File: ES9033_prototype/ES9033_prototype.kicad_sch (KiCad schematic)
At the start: 8 parts, among them J101 Conn_01x02, J102 Conn_01x04, J103 Conn_01x04, J104 Conn_01x04

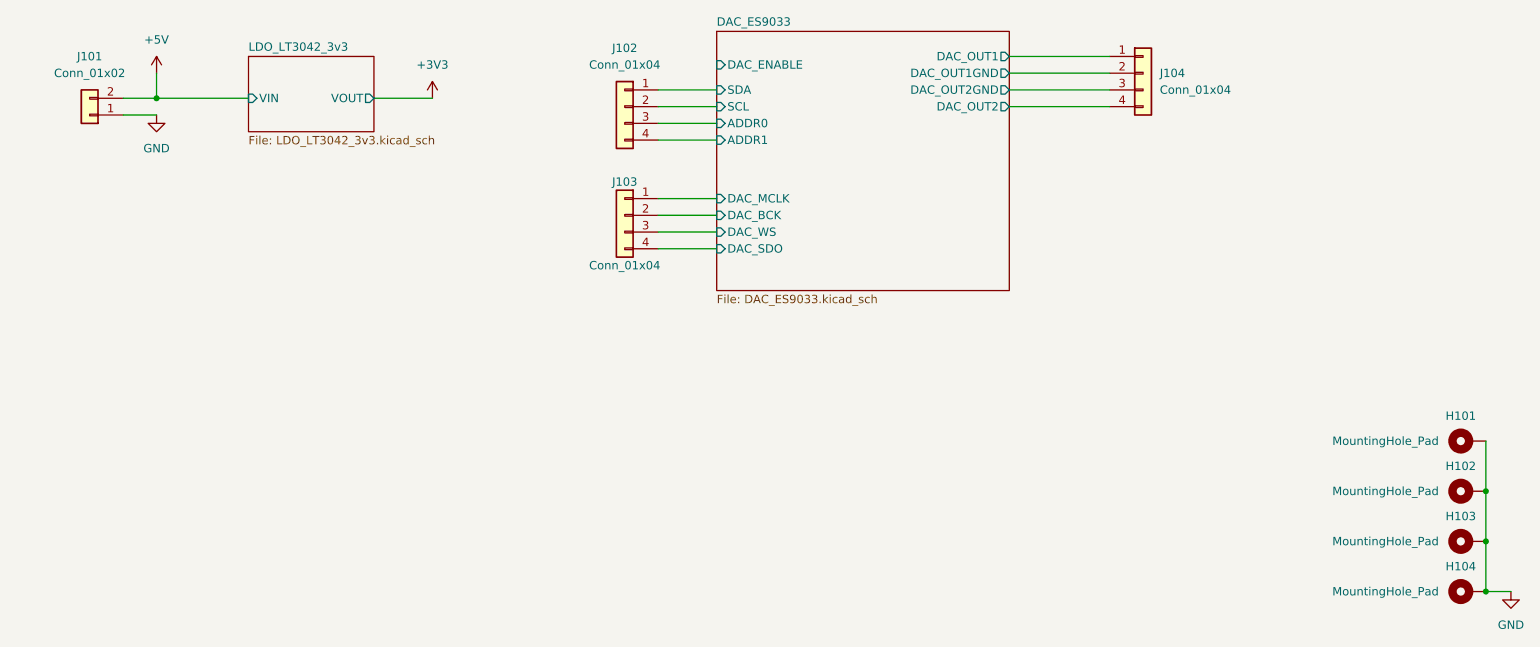
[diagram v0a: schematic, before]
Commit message: changed header
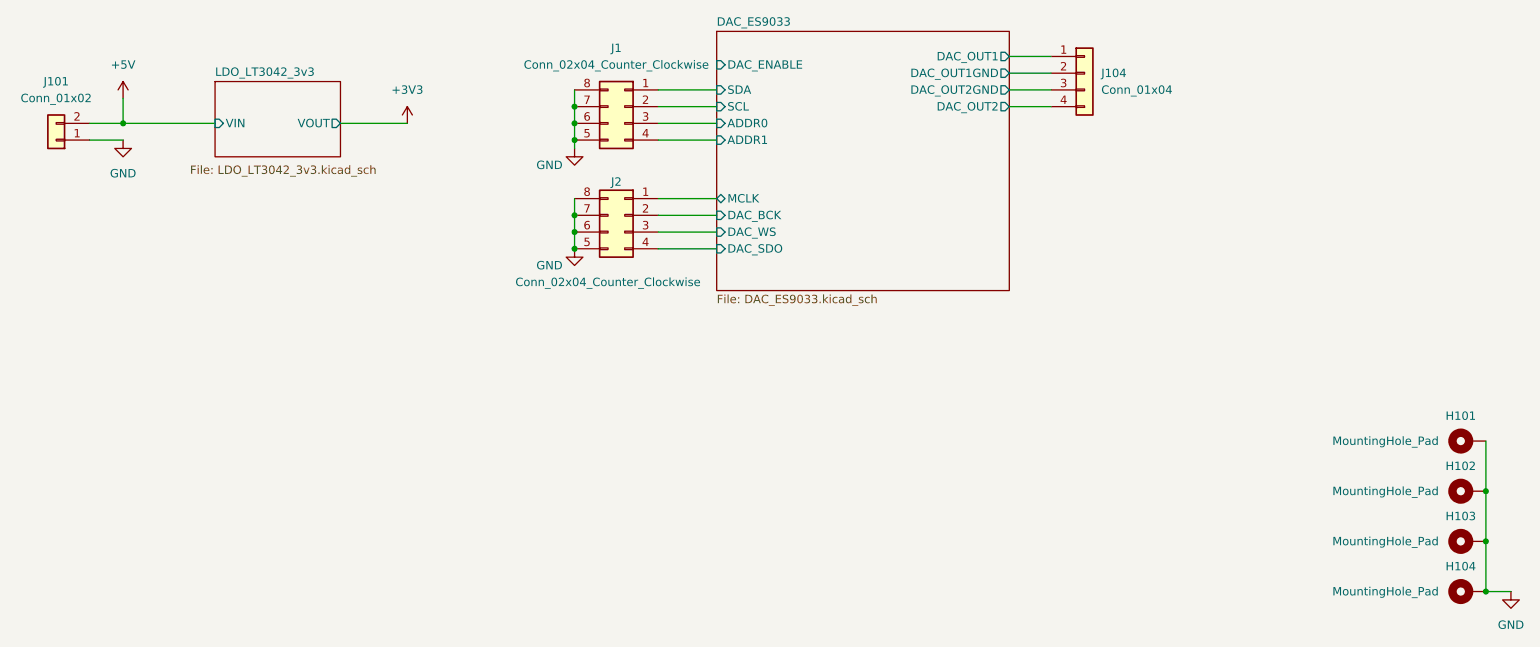
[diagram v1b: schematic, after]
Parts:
- removed J102, J103: Conn_01x04, Connector_PinHeader_2.54mm:PinHeader_1x04_P2.54mm_Vertical, symbol Connector_Generic:Conn_01x04
- added J1, J2: Conn_02x04_Counter_Clockwise, Connector_PinHeader_2.54mm:PinHeader_2x04_P2.54mm_Vertical, symbol Connector_Generic:Conn_02x04_Counter_Clockwise
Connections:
- net DAC_ES9033/ADDR0: now also J1.3 (Pin_3)
- net DAC_ES9033/ADDR1: now also J1.4 (Pin_4)
- net DAC_ES9033/DAC_BCK: now also J2.2 (Pin_2)
- net DAC_ES9033/DAC_SDO: now also J2.4 (Pin_4)
- net DAC_ES9033/DAC_WS: now also J2.3 (Pin_3)
- net DAC_ES9033/SCL: now also J1.2 (Pin_2)
- net DAC_ES9033/SDA: now also J1.1 (Pin_1)
- net GND: now also J1.5 (Pin_5), J1.6 (Pin_6), J1.7 (Pin_7), J1.8 (Pin_8), J2.5 (Pin_5), J2.6 (Pin_6), J2.7 (Pin_7), J2.8 (Pin_8)
- new net DAC_ES9033/MCLK: J2.1 (Pin_1)
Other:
- sheet DAC_ES9033 ports: added MCLK; removed DAC_MCLK
- moved on the sheet: J101, J104
